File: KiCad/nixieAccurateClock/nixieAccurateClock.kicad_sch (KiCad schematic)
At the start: 9 parts, among them J2 Conn_02x20_Odd_Even, J3 Conn_02x20_Odd_Even, J3 Conn_Coaxial, U1 PX1125T

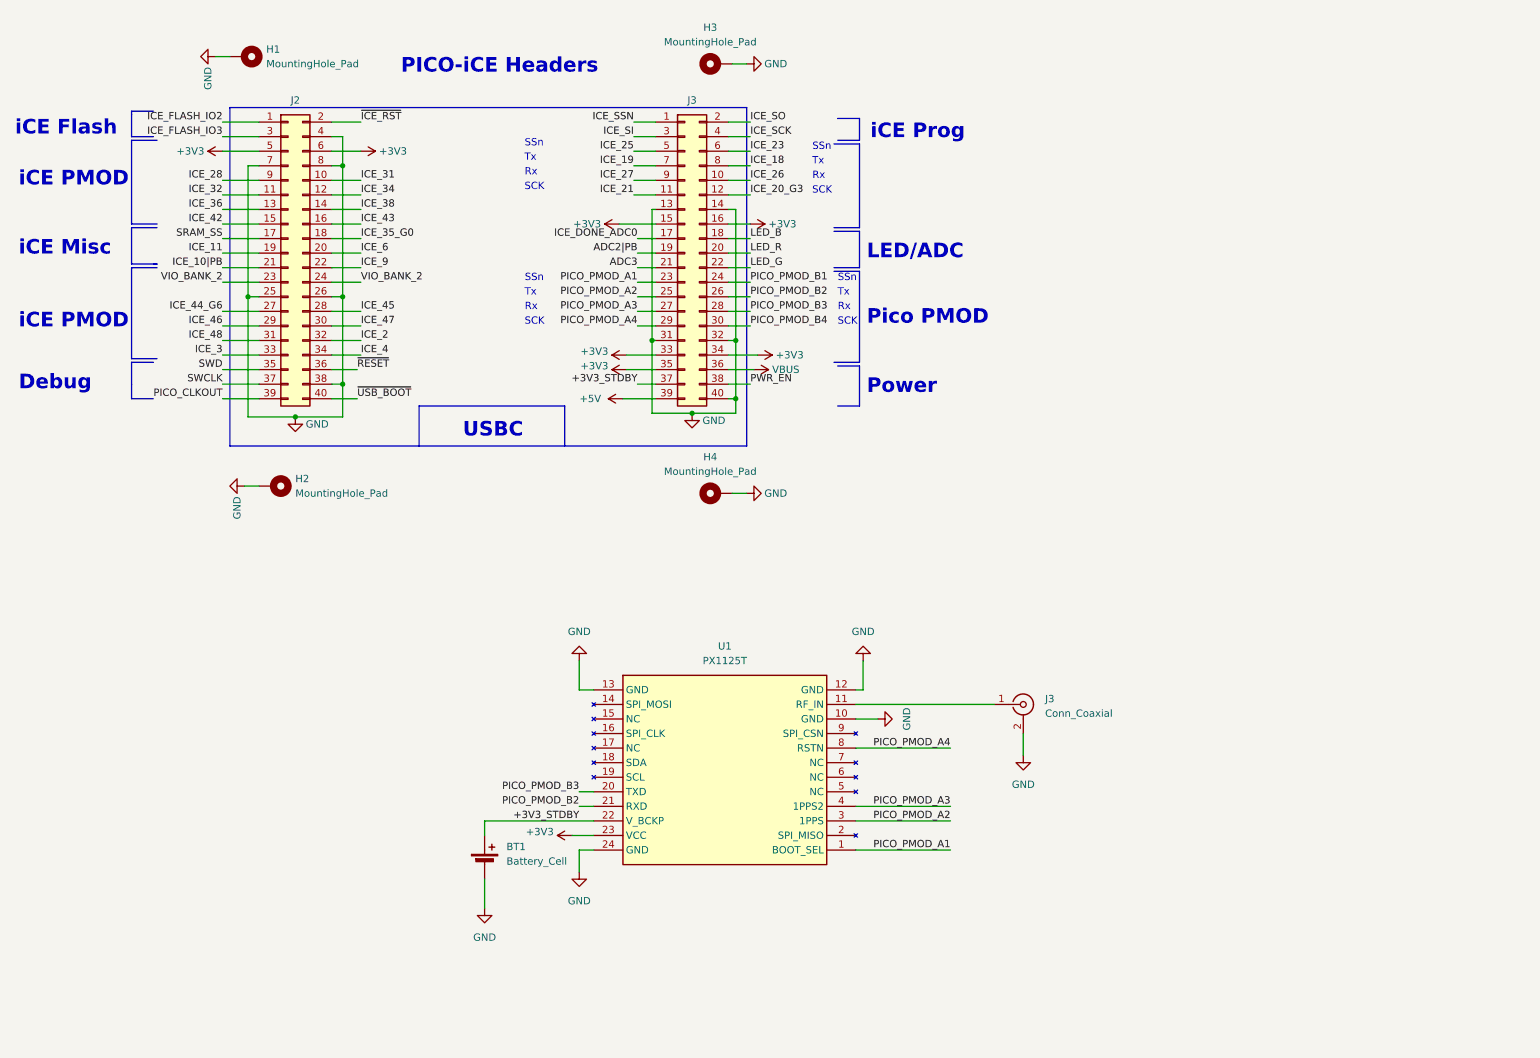
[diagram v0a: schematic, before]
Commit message: Add high voltage supply
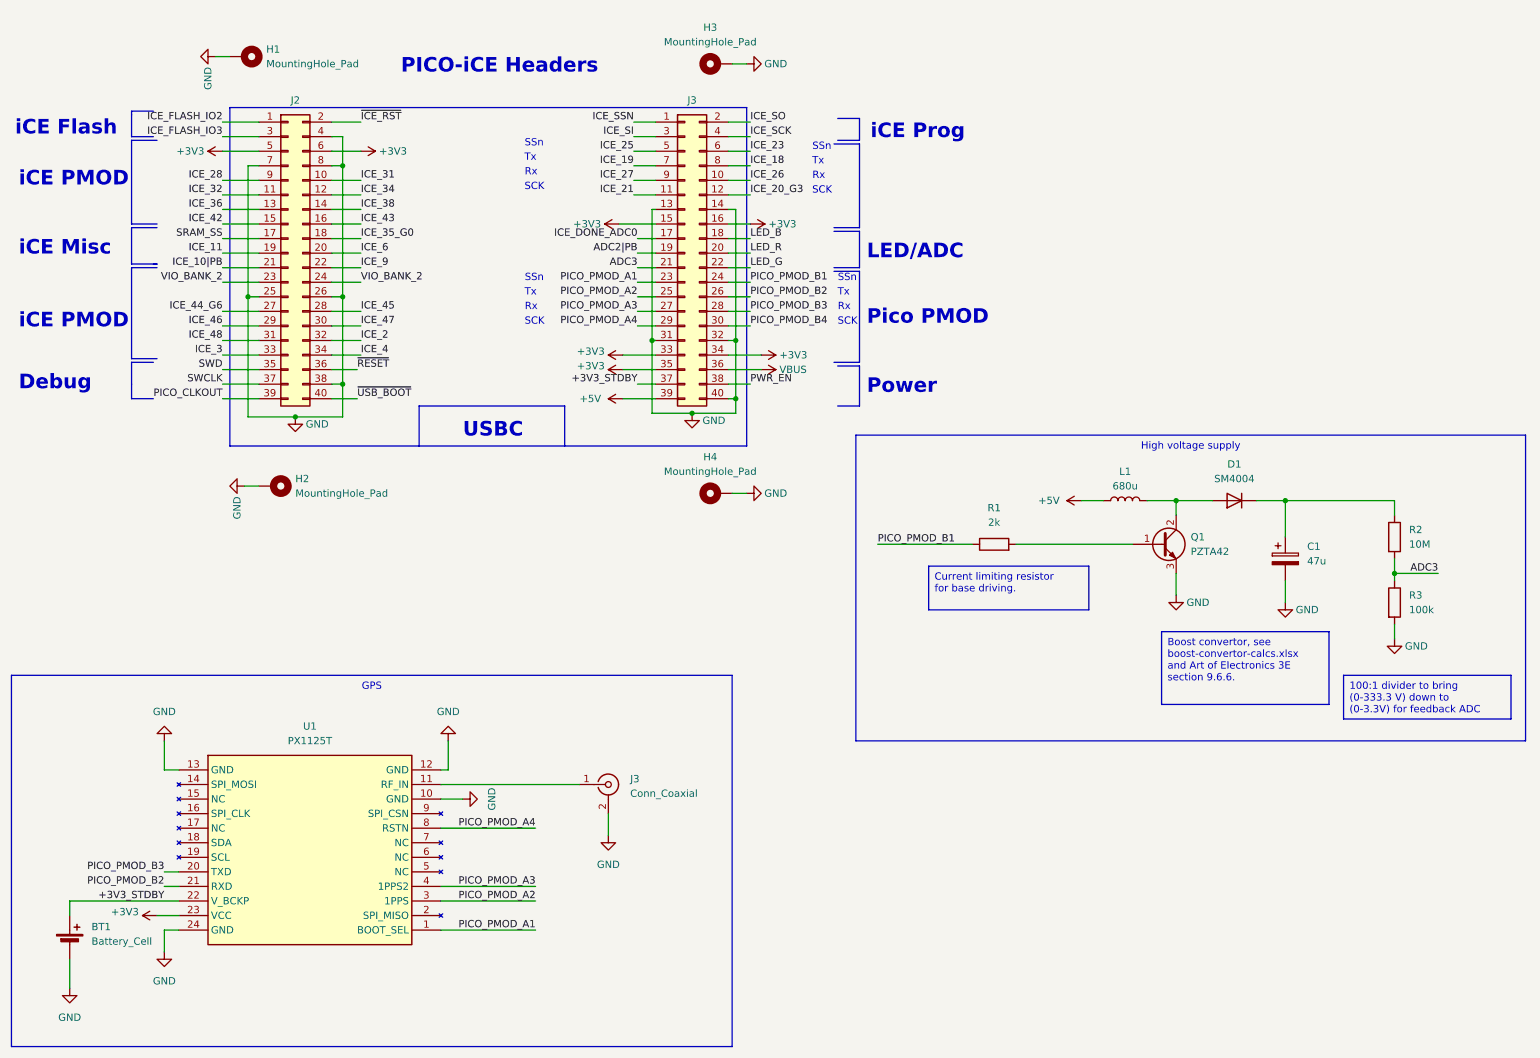
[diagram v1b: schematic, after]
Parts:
- added C1: 47u, Capacitor_THT:C_Radial_D12.5mm_H20.0mm_P5.00mm, symbol Device:C_Polarized
- added D1: SM4004, Diode_SMD:D_MELF, symbol Diode:SM4004
- added L1: 680u, 00_lib:IND_MSS1583_COC, symbol Device:L
- added Q1: PZTA42, Package_TO_SOT_SMD:SOT-223-3_TabPin2, symbol Transistor_BJT:PZTA42
- added R1: 2k, Resistor_SMD:R_0603_1608Metric, symbol Device:R
- added R2: 10M, Resistor_SMD:R_0603_1608Metric, symbol Device:R
- added R3: 100k, Resistor_SMD:R_0603_1608Metric, symbol Device:R
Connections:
- net +5V: now also L1.1
- net ADC3: now also R2.2, R3.1
- net GND: now also C1.2, Q1.3 (E), R3.2
- net PICO_PMOD_B1: now also R1.1
- new net: D1.2 (A), L1.2, Q1.2 (C)
- new net: C1.1, D1.1 (K), R2.1
- new net: Q1.1 (B), R1.2
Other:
- moved on the sheet: BT1, J3, U1

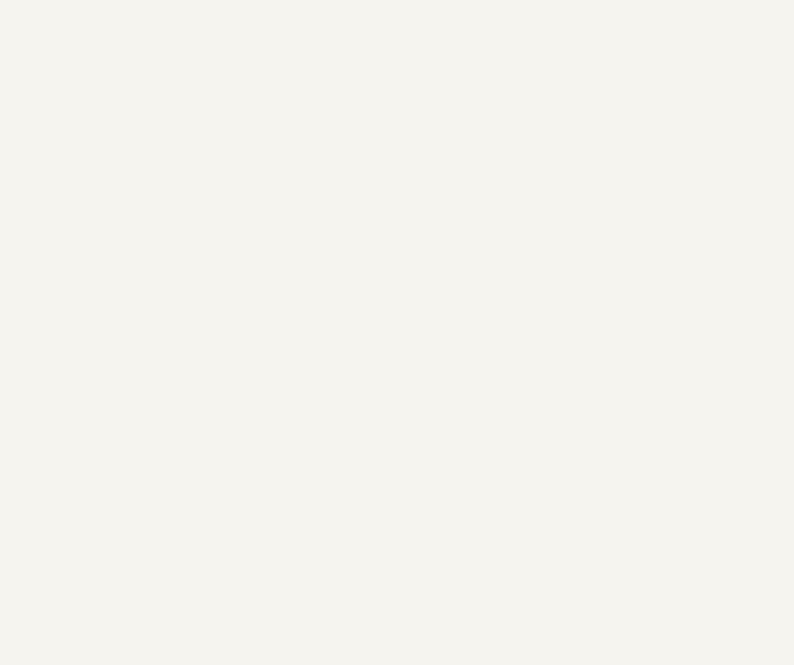
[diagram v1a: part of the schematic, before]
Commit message: Add DST controlling DIP switches
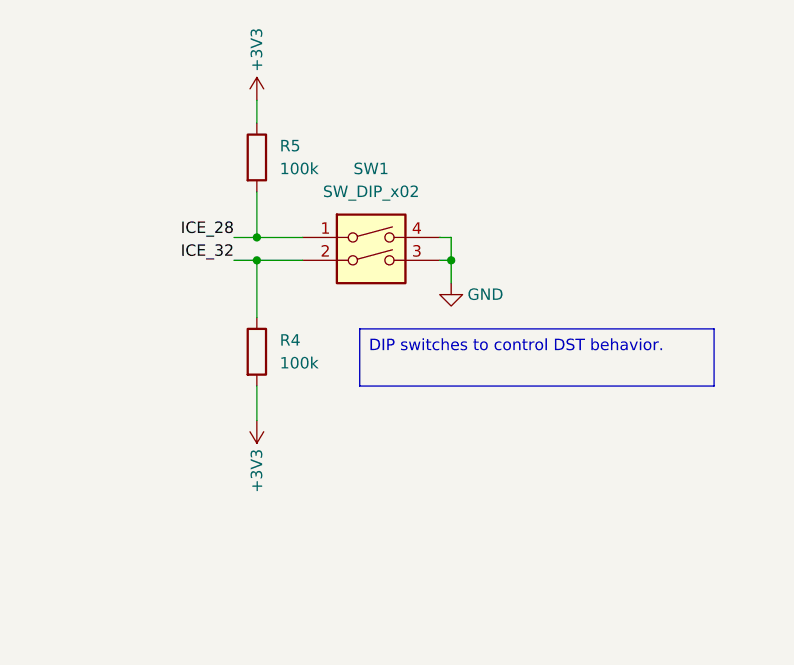
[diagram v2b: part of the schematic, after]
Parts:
- added R4, R5: 100k, Resistor_SMD:R_0603_1608Metric, symbol Device:R
- added SW1: SW_DIP_x02, Button_Switch_THT:SW_DIP_SPSTx02_Slide_6.7x6.64mm_W7.62mm_P2.54mm_LowProfile, symbol Switch:SW_DIP_x02
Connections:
- net +3V3: now also R4.2, R5.1
- net GND: now also SW1.3, SW1.4
- net ICE_28: now also R5.2, SW1.1
- net ICE_32: now also R4.1, SW1.2
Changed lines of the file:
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@@
   (junction (at 220.98 97.79) (diameter 0) (color 0 0 0 0)
   )
+  (junction (at 224.79 39.37) (diameter 0) (color 0 0 0 0)
+  )
   (junction (at 75.565 62.23) (diameter 0) (color 0 0 0 0)
   )
@@
   (junction (at 144.145 80.01) (diameter 0) (color 0 0 0 0)
   )
+  (junction (at 246.38 39.37) (diameter 0) (color 0 0 0 0)
+  )
   (junction (at 259.08 110.49) (diameter 0) (color 0 0 0 0)
   )
   (junction (at 144.145 69.85) (diameter 0) (color 0 0 0 0)
   )
+  (junction (at 224.79 36.83) (diameter 0) (color 0 0 0 0)
+  )
   (junction (at 75.565 77.47) (diameter 0) (color 0 0 0 0)
   )
@@
     (stroke (width 0) (type default))
   )
+  (wire (pts (xy 224.79 36.83) (xy 229.87 36.83))
+    (stroke (width 0) (type default))
+  )
   (wire (pts (xy 130.175 62.23) (xy 127 62.23))
     (stroke (width 0) (type default))
@@
     (stroke (width 0) (type default))
   )
+  (wire (pts (xy 222.25 36.83) (xy 224.79 36.83))
+    (stroke (width 0) (type default))
+  )
   (wire (pts (xy 92.71 172.72) (xy 109.22 172.72))
     (stroke (width 0) (type default))
@@
     (stroke (width 0) (type default))
   )
+  (wire (pts (xy 245.11 36.83) (xy 246.38 36.83))
+    (stroke (width 0) (type default))
+  )
   (polyline (pts (xy 38.735 57.15) (xy 38.735 73.025))
     (stroke (width 0) (type default))
@@
     (stroke (width 0) (type default))
   )
+  (wire (pts (xy 224.79 53.34) (xy 224.79 57.15))
+    (stroke (width 0) (type default))
+  )
   (polyline (pts (xy 165.735 35.56) (xy 161.29 35.56))
     (stroke (width 0) (type default))
   )
+  (wire (pts (xy 224.79 39.37) (xy 224.79 45.72))
+    (stroke (width 0) (type default))
+  )
   (polyline (pts (xy 161.925 74.295) (xy 165.735 74.295))
     (stroke (width 0) (type default))
   )
+  (wire (pts (xy 246.38 36.83) (xy 246.38 39.37))
+    (stroke (width 0) (type default))
+  )
   (wire (pts (xy 124.46 80.01) (xy 130.175 80.01))
     (stroke (width 0) (type default))
@@
     (stroke (width 0) (type default))
   )
+  (wire (pts (xy 245.11 39.37) (xy 246.38 39.37))
+    (stroke (width 0) (type default))
+  )
   (wire (pts (xy 54.61 31.75) (xy 60.96 31.75))
     (stroke (width 0) (type default))
@@
     (stroke (width 0) (type default))
   )
+  (wire (pts (xy 222.25 39.37) (xy 224.79 39.37))
+    (stroke (width 0) (type default))
+  )
+  (wire (pts (xy 246.38 39.37) (xy 246.38 41.91))
+    (stroke (width 0) (type default))
+  )
   (wire (pts (xy 73.66 69.85) (xy 78.74 69.85))
     (stroke (width 0) (type default))
@@
     (stroke (width 0) (type default))
   )
+  (wire (pts (xy 224.79 21.59) (xy 224.79 24.13))
+    (stroke (width 0) (type default))
+  )
   (wire (pts (xy 78.74 41.91) (xy 73.66 41.91))
     (stroke (width 0) (type default))
@@
     (stroke (width 0) (type default))
   )
+  (wire (pts (xy 229.87 39.37) (xy 224.79 39.37))
+    (stroke (width 0) (type default))
+  )
   (wire (pts (xy 129.54 69.85) (xy 129.54 46.99))
     (stroke (width 0) (type default))
@@
   )
   (wire (pts (xy 127 52.07) (xy 130.175 52.07))
+    (stroke (width 0) (type default))
+  )
+  (wire (pts (xy 224.79 31.75) (xy 224.79 36.83))
     (stroke (width 0) (type default))
   )
@@
     (effects (font (size 1.27 1.27)) (justify left top))
   )
+  (text_box "DIP switches to control DST behavior."
+    (at 236.22 46.99 0) (size 39.37 6.35)
+    (stroke (width 0) (type default))
+    (fill (type none))
+    (effects (font (size 1.27 1.27)) (justify left top))
+  )
   (text_box "GPS"
     (at 17.78 128.27 0) (size 125.73 64.77)
@@
     (effects (font (size 1.27 1.27)) (justify right bottom))
   )
+  (label "ICE_28" (at 222.25 36.83 180) (fields_autoplaced)
+    (effects (font (size 1.27 1.27)) (justify right bottom))
+  )
   (label "ICE_47" (at 78.74 67.31 0) (fields_autoplaced)
     (effects (font (size 1.27 1.27)) (justify left bottom))
@@
   )
   (label "ICE_44_G6" (at 54.61 64.77 180) (fields_autoplaced)
+    (effects (font (size 1.27 1.27)) (justify right bottom))
+  )
+  (label "ICE_32" (at 222.25 39.37 180) (fields_autoplaced)
     (effects (font (size 1.27 1.27)) (justify right bottom))
   )
@@
         (path "/55aab698-7558-4fe2-95ad-faa6da60ef89"
           (reference "H1") (unit 1)
+        )
+      )
+    )
+  )
+  (symbol (lib_id "power:+3V3") (at 224.79 21.59 0) (unit 1)
+    (in_bom yes) (on_board yes) (dnp no)
+    (property "Reference" "#PWR034" (at 224.79 25.4 0)
+      (effects (font (size 1.27 1.27)) hide)
+    )
+    (property "Value" "+3V3" (at 224.79 18.415 90)
+      (effects (font (size 1.27 1.27)) (justify left))
+    )
+    (property "Footprint" "" (at 224.79 21.59 0)
+      (effects (font (size 1.27 1.27)) hide)
+    )
+    (property "Datasheet" "" (at 224.79 21.59 0)
+      (effects (font (size 1.27 1.27)) hide)
+    )
+    (pin "1")
+    (instances
+      (project "pico-ice"
+        (path "/2ff44921-0562-495a-89f5-ac439f192d90"
+          (reference "#PWR034") (unit 1)
+        )
+      )
+      (project "nixieAccurateClock"
+        (path "/55aab698-7558-4fe2-95ad-faa6da60ef89"
+          (reference "#PWR027") (unit 1)
         )
       )
@@
     )
   )
+  (symbol (lib_id "power:GND") (at 246.38 41.91 0) (mirror y) (unit 1)
+    (in_bom yes) (on_board yes) (dnp no)
+    (property "Reference" "#PWR059" (at 246.38 48.26 0)
+      (effects (font (size 1.27 1.27)) hide)
+    )
+    (property "Value" "GND" (at 250.19 43.18 0)
+      (effects (font (size 1.27 1.27)))
+    )
+    (property "Footprint" "" (at 246.38 41.91 0)
+      (effects (font (size 1.27 1.27)) hide)
+    )
+    (property "Datasheet" "" (at 246.38 41.91 0)
+      (effects (font (size 1.27 1.27)) hide)
+    )
+    (pin "1")
+    (instances
+      (project "pico-ice"
+        (path "/2ff44921-0562-495a-89f5-ac439f192d90"
+          (reference "#PWR059") (unit 1)
+        )
+      )
+      (project "nixieAccurateClock"
+        (path "/55aab698-7558-4fe2-95ad-faa6da60ef89"
+          (reference "#PWR029") (unit 1)
+        )
+      )
+    )
+  )
   (symbol (lib_id "power:+3V3") (at 78.74 36.83 270) (unit 1)
     (in_bom yes) (on_board yes) (dnp no)
@@
     )
   )
+  (symbol (lib_id "Device:R") (at 224.79 49.53 0) (unit 1)
+    (in_bom yes) (on_board yes) (dnp no) (fields_autoplaced)
+    (property "Reference" "R4" (at 227.33 48.26 0)
+      (effects (font (size 1.27 1.27)) (justify left))
+    )
+    (property "Value" "100k" (at 227.33 50.8 0)
+      (effects (font (size 1.27 1.27)) (justify left))
+    )
+    (property "Footprint" "Resistor_SMD:R_0603_1608Metric" (at 223.012 49.53 90)
+      (effects (font (size 1.27 1.27)) hide)
+    )
+    (property "Datasheet" "~" (at 224.79 49.53 0)
+      (effects (font (size 1.27 1.27)) hide)
+    )
+    (pin "1")
+    (pin "2")
+    (instances
+      (project "nixieAccurateClock"
+        (path "/55aab698-7558-4fe2-95ad-faa6da60ef89"
+          (reference "R4") (unit 1)
+        )
+      )
+    )
+  )
+  (symbol (lib_id "power:+3V3") (at 224.79 57.15 180) (unit 1)
+    (in_bom yes) (on_board yes) (dnp no)
+    (property "Reference" "#PWR034" (at 224.79 53.34 0)
+      (effects (font (size 1.27 1.27)) hide)
+    )
+    (property "Value" "+3V3" (at 224.79 60.325 90)
+      (effects (font (size 1.27 1.27)) (justify left))
+    )
+    (property "Footprint" "" (at 224.79 57.15 0)
+      (effects (font (size 1.27 1.27)) hide)
+    )
+    (property "Datasheet" "" (at 224.79 57.15 0)
+      (effects (font (size 1.27 1.27)) hide)
+    )
+    (pin "1")
+    (instances
+      (project "pico-ice"
+        (path "/2ff44921-0562-495a-89f5-ac439f192d90"
+          (reference "#PWR034") (unit 1)
+        )
+      )
+      (project "nixieAccurateClock"
+        (path "/55aab698-7558-4fe2-95ad-faa6da60ef89"
+          (reference "#PWR028") (unit 1)
+        )
+      )
+    )
+  )
   (symbol (lib_name "GND_1") (lib_id "power:GND") (at 93.98 139.7 0) (mirror x) (unit 1)
     (in_bom yes) (on_board yes) (dnp no)
@@
     )
   )
+  (symbol (lib_id "Switch:SW_DIP_x02") (at 237.49 39.37 0) (unit 1)
+    (in_bom yes) (on_board yes) (dnp no) (fields_autoplaced)
+    (property "Reference" "SW1" (at 237.49 29.21 0)
+      (effects (font (size 1.27 1.27)))
+    )
+    (property "Value" "SW_DIP_x02" (at 237.49 31.75 0)
+      (effects (font (size 1.27 1.27)))
+    )
+    (property "Footprint" "Button_Switch_THT:SW_DIP_SPSTx02_Slide_6.7x6.64mm_W7.62mm_P2.54mm_LowProfile" (at 237.49 39.37 0)
+      (effects (font (size 1.27 1.27)) hide)
+    )
+    (property "Datasheet" "https://www.mouser.com/datasheet/2/670/ds02_254-1777565.pdf" (at 237.49 39.37 0)
+      (effects (font (size 1.27 1.27)) hide)
+    )
+    (property "Model" "DS02-254-1L-02BE" (at 237.49 39.37 0)
+      (effects (font (size 1.27 1.27)) hide)
+    )
+    (pin "1")
+    (pin "4")
+    (pin "3")
+    (pin "2")
+    (instances
+      (project "nixieAccurateClock"
+        (path "/55aab698-7558-4fe2-95ad-faa6da60ef89"
+          (reference "SW1") (unit 1)
+        )
+      )
+    )
+  )
   (symbol (lib_id "power:+3V3") (at 148.59 72.39 270) (mirror x) (unit 1)
     (in_bom yes) (on_board yes) (dnp no)
@@
         )
       )
+    )
+  )
+  (symbol (lib_id "Device:R") (at 224.79 27.94 0) (unit 1)
+    (in_bom yes) (on_board yes) (dnp no) (fields_autoplaced)
+    (property "Reference" "R5" (at 227.33 26.67 0)
+      (effects (font (size 1.27 1.27)) (justify left))
+    )
+    (property "Value" "100k" (at 227.33 29.21 0)
+      (effects (font (size 1.27 1.27)) (justify left))
+    )
+    (property "Footprint" "Resistor_SMD:R_0603_1608Metric" (at 223.012 27.94 90)
+      (effects (font (size 1.27 1.27)) hide)
+    )
+    (property "Datasheet" "~" (at 224.79 27.94 0)
+      (effects (font (size 1.27 1.27)) hide)
+    )
+    (pin "1")
+    (pin "2")
+    (instances
+      (project "nixieAccurateClock"
+        (path "/55aab698-7558-4fe2-95ad-faa6da60ef89"
+          (reference "R5") (unit 1)
+        )
+      )
